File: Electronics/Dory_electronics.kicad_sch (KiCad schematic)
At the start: 21 parts, among them J1 Bateria 2S, J10 SHARP_CENTRO_E, J2 Conn_01x08, J3 Conn_01x08, J4 Motor B, J5 Motor A, J6 sensor IR, J7 VL53L0X_ESQUERDO, J8 SHARP_CENTRO_D, J9 VL53L0X_DIREITO, SW1 SW_Push, U1 LM1117 5V

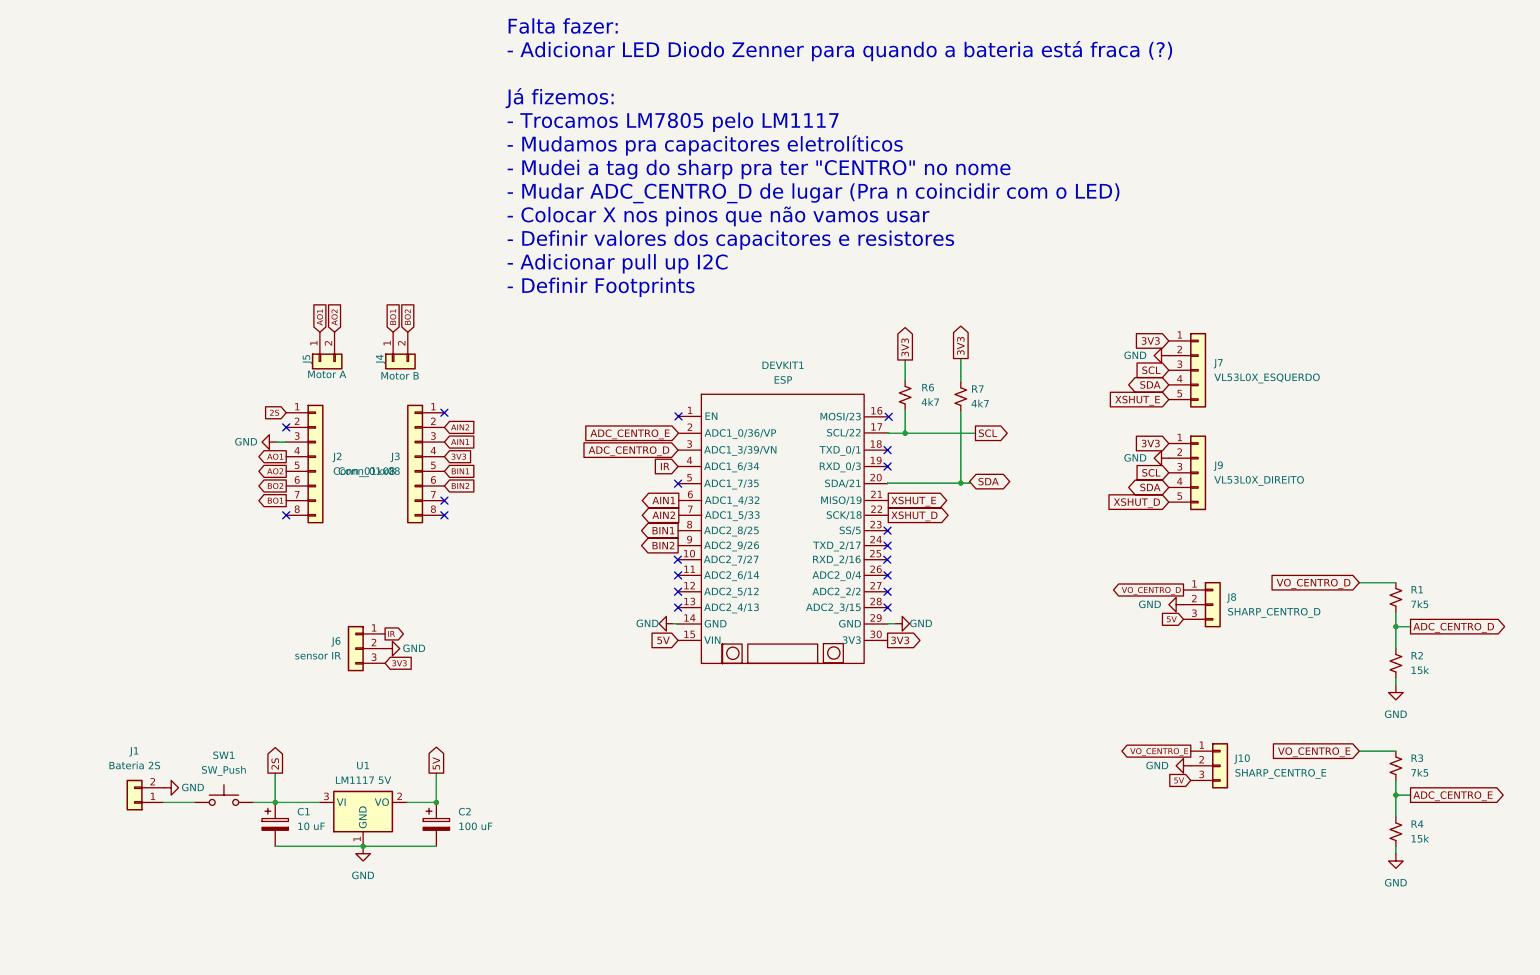
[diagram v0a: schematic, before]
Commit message: chore(Electronics): organize and finish schematic
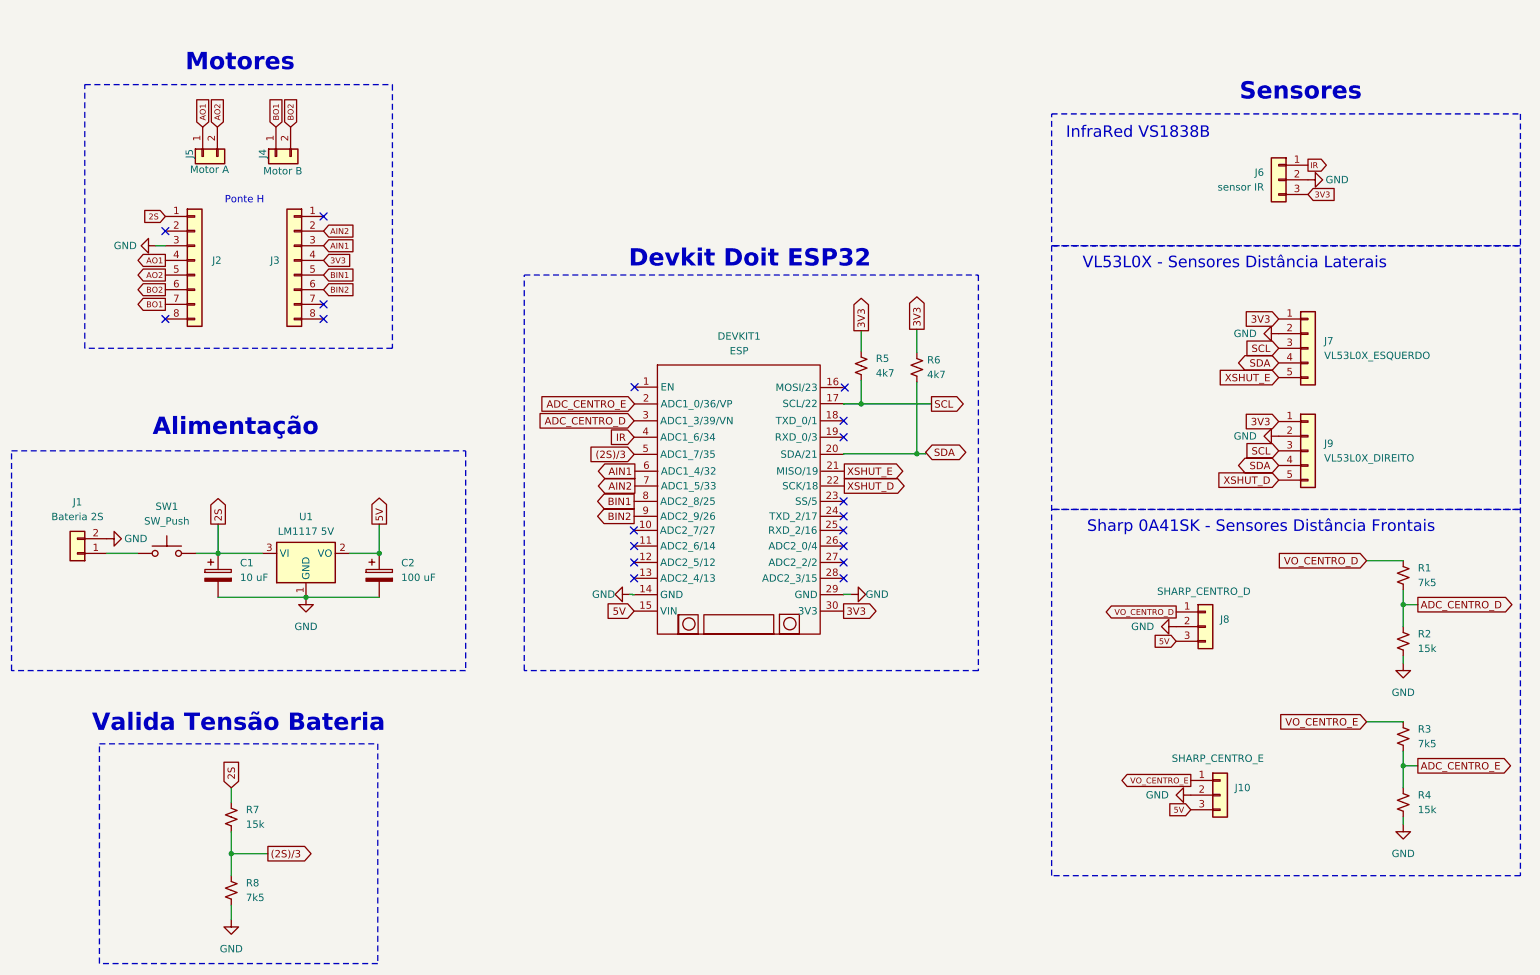
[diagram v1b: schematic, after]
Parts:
- added R7: 15k, Resistor_SMD:R_0805_2012Metric, symbol Device:R_Small_US
- added R8: 7k5, Resistor_SMD:R_0805_2012Metric, symbol Device:R_Small_US
- DEVKIT1: footprint KIKAD bibliotecas:esp32_devkit_v1_doit -> esp32_devkit_v1_doit:esp32_devkit_v1_doit
- renumbered R6 to R5, R7 to R6
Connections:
- net 2S: now also R7.1
- net GND: now also R8.2
- net (2S)/3: now reaches DEVKIT1.5 (ADC1_7/35)
- net (2S)/3: now also R7.2, R8.1
- no-connect marks 20 -> 19
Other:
- note added: "Alimentação"
- note added: "Devkit Doit ESP32"
- note added: "InfraRed VS1838B"
- note added: "Motores"
- note added: "Ponte H"
- note added: "Sensores"
- note added: "Sharp 0A41SK - Sensores Distância Frontais"
- note added: "VL53L0X - Sensores Distância Laterais"
- note added: "Valida Tensão Bateria"
- note removed: "Falta fazer: - Adicionar LED Diodo Zenner para quando a bateria está fraca (?) Já fizemos: - Trocamos LM7805 pelo LM1117 - Mudamos pra capacitores eletrolíticos - Mudei a tag do sharp pra ter "CENTRO" no nome - Mudar ADC_CENTRO_D de lugar (Pra n coincidir com o LED) - Colocar X nos pinos que não vamos usar - Definir valores dos capacitores e resistores - Adicionar pull up I2C - Definir Footprints"
- moved on the sheet: C1, C2, DEVKIT1, J1, J10, J2, J3, J4, J5, J6, J7, J8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
